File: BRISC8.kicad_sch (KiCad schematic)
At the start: 0 parts

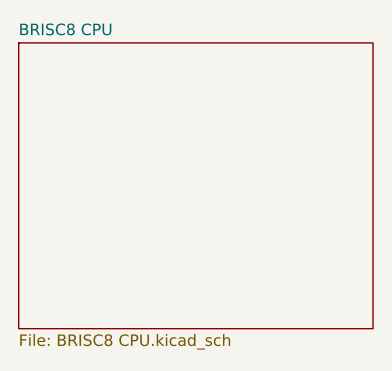
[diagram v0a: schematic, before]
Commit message: Fixed(?)
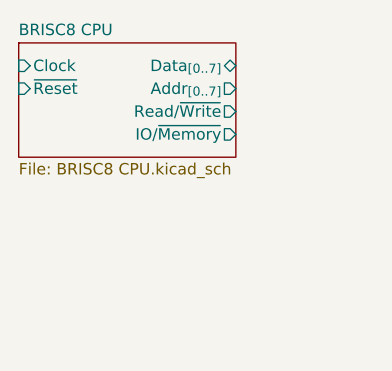
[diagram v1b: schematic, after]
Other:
- sheet BRISC8 CPU ports: added Addr_{[0..7]}, Clock, Data_{[0..7]}, IO/~{Memory}, Read/~{Write}, ~{Reset}; removed none
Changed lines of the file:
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@@
 	(sheet
 		(at 93.98 53.34)
-		(size 39.37 31.75)
+		(size 24.13 12.7)
 		(exclude_from_sim no)
 		(in_bom yes)
@@
 		)
 		(property "Sheetfile" "BRISC8 CPU.kicad_sch"
-			(at 93.98 85.6746 0)
+			(at 93.98 66.6246 0)
 			(effects
 				(font
@@
 			)
 		)
+		(pin "Data_{[0..7]}" bidirectional
+			(at 118.11 55.88 0)
+			(effects
+				(font
+					(size 1.27 1.27)
+				)
+				(justify right)
+			)
+		)
+		(pin "Addr_{[0..7]}" output
+			(at 118.11 58.42 0)
+			(effects
+				(font
+					(size 1.27 1.27)
+				)
+				(justify right)
+			)
+		)
+		(pin "Read{slash}~{Write}" output
+			(at 118.11 60.96 0)
+			(effects
+				(font
+					(size 1.27 1.27)
+				)
+				(justify right)
+			)
+		)
+		(pin "IO{slash}~{Memory}" output
+			(at 118.11 63.5 0)
+			(effects
+				(font
+					(size 1.27 1.27)
+				)
+				(justify right)
+			)
+		)
+		(pin "Clock" input
+			(at 93.98 55.88 180)
+			(effects
+				(font
+					(size 1.27 1.27)
+				)
+				(justify left)
+			)
+		)
+		(pin "~{Reset}" input
+			(at 93.98 58.42 180)
+			(effects
+				(font
+					(size 1.27 1.27)
+				)
+				(justify left)
+			)
+		)
